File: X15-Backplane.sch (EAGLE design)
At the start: 35 parts

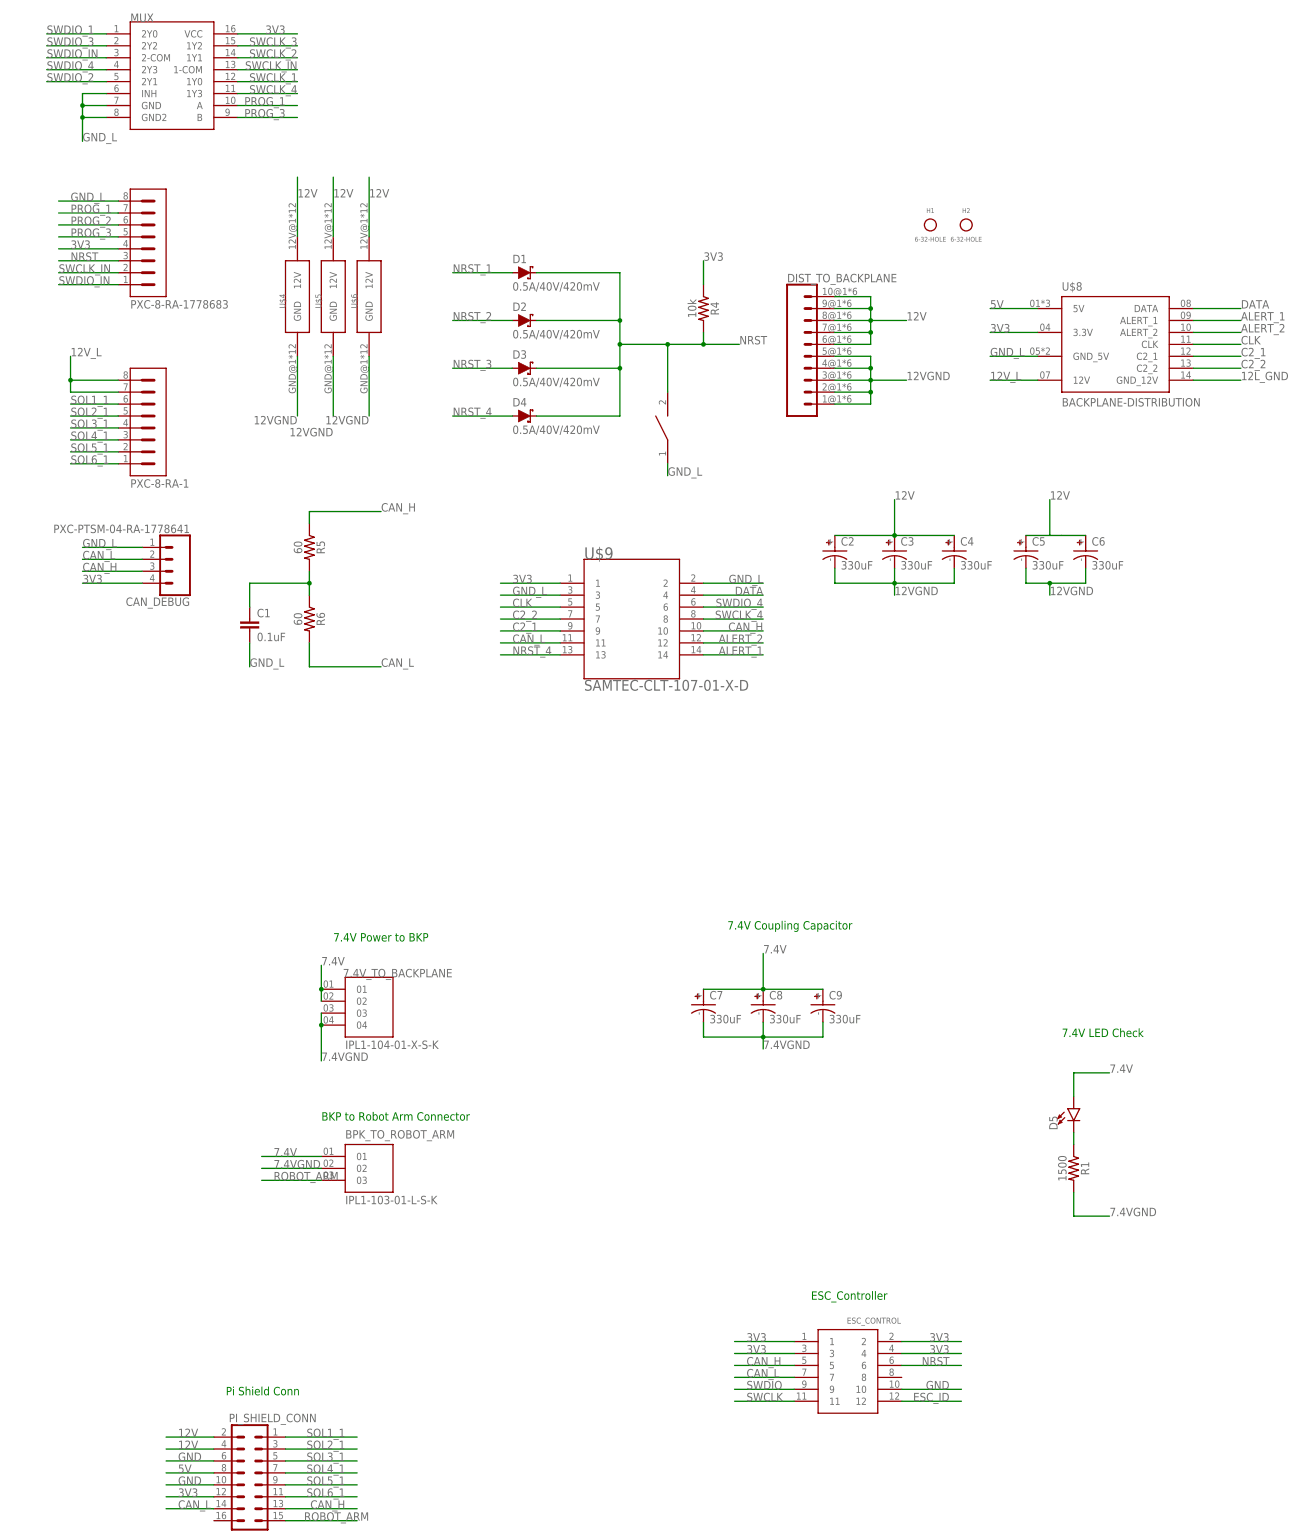
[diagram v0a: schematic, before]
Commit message: Backplane
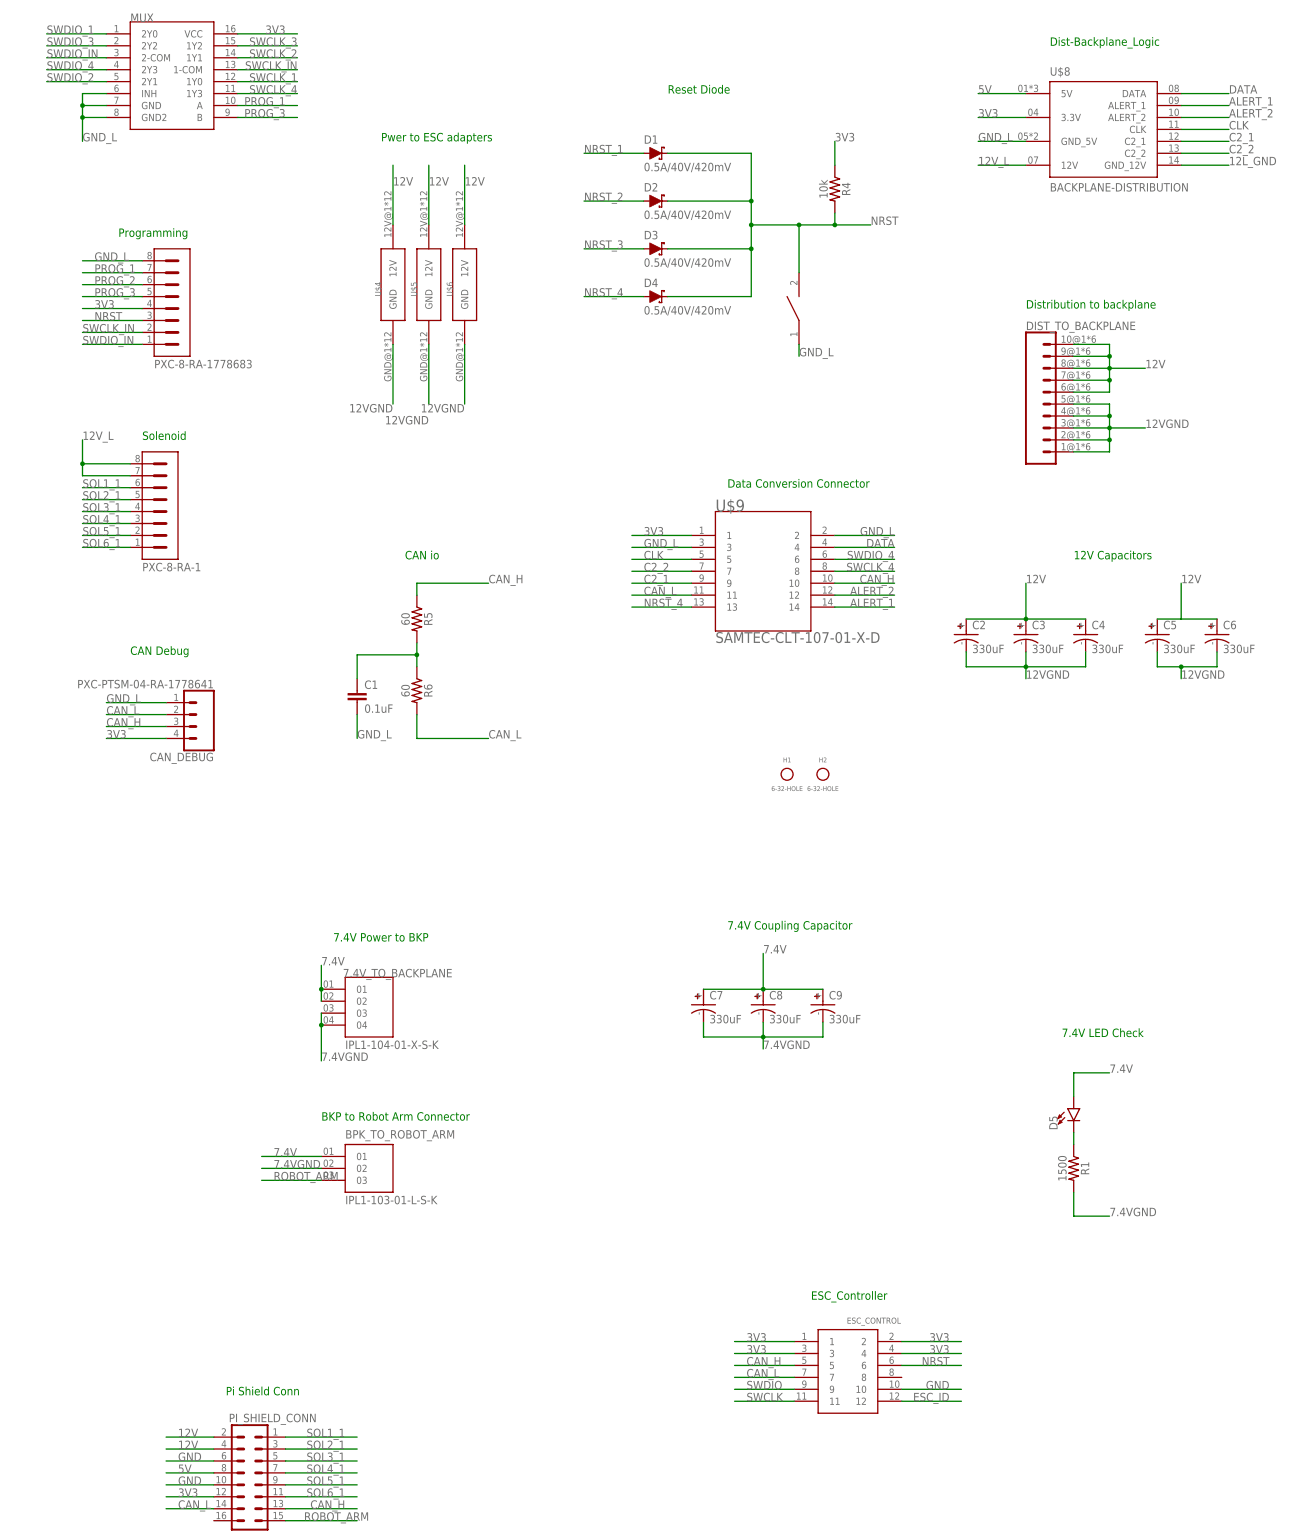
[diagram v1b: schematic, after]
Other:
- note added: "12V Capacitors"
- note added: "CAN Debug"
- note added: "CAN io"
- note added: "Data Conversion Connector"
- note added: "Dist-Backplane_Logic"
- note added: "Distribution to backplane"
- note added: "Programming"
- note added: "Pwer to ESC adapters"
- note added: "Reset Diode"
- note added: "Solenoid"
- moved on the sheet: C1, C2, C3, C4, C5, C6, CAN_DEBUG, D1, D2, D3, D4, DIST_TO_BACKPLANE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
